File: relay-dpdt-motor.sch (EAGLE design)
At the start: 4 parts, among them K1 4052

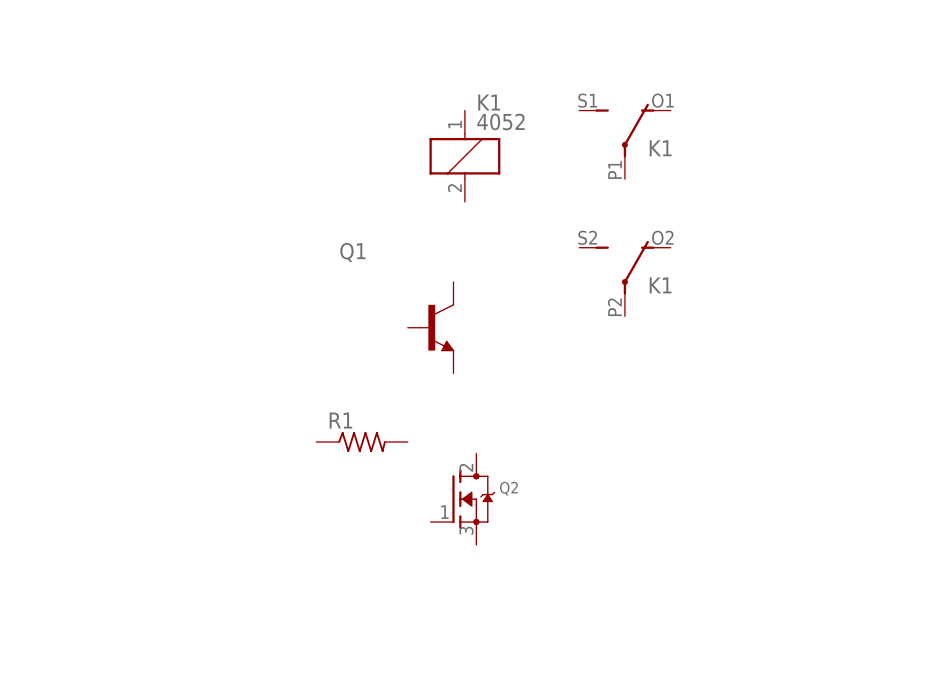
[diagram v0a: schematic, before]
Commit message: eagle prewired
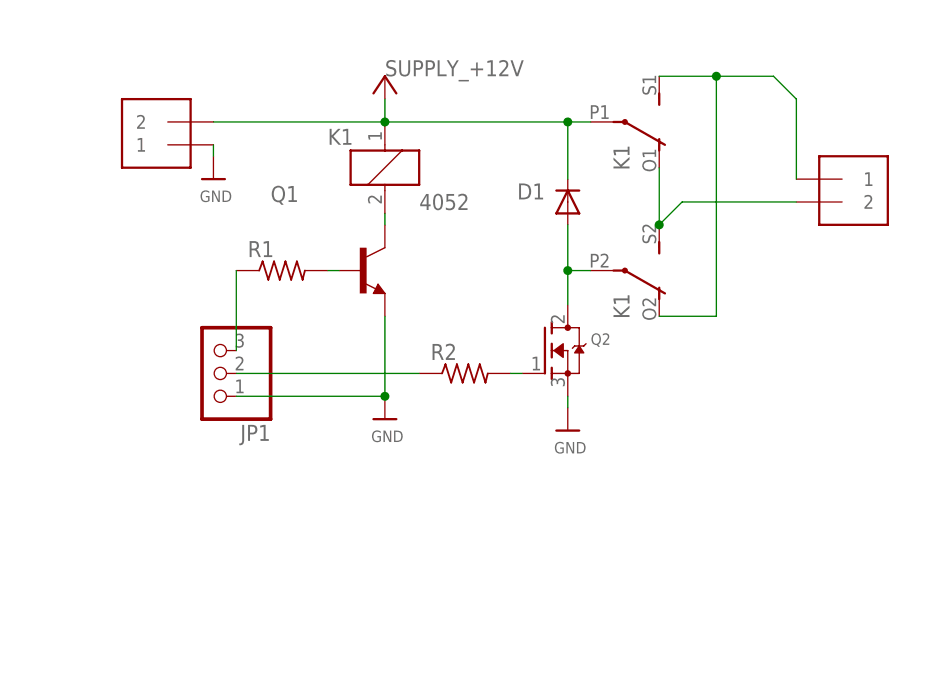
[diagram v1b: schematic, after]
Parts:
- added D1: 1N4004, adafruit:1N4004
- added J1, J2: 1X2-3.5MM, adafruit:1X2-3.5MM
- added JP1: (no value), adafruit:PINHD-1X3CB
- added R2: (no value), adafruit:R-US_0204/7
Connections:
- new net +12V: D1.C, J1.2, K11.1, K12.P
- new net GND: J1.1, JP1.1, Q1.E, Q2.S
- new net N$1: Q1.B, R1.2
- new net N$2: K11.2, Q1.C
- new net N$3: Q2.G, R2.2
- new net N$5: D1.A, K13.P, Q2.D
- new net N$6: J2.1, K12.S, K13.O
- new net N$7: J2.2, K12.O, K13.S
- new net N$8: JP1.2, R2.1
- new net N$9: JP1.3, R1.1
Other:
- moved on the sheet: K1, Q1, Q2, R1
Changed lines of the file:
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@@
 <setting verticaltext="up"/>
 </settings>
-<grid distance="0.1" unitdist="inch" unit="inch" style="lines" multiple="1" display="no" altdistance="0.01" altunitdist="inch" altunit="inch"/>
+<grid distance="50" unitdist="mil" unit="mil" style="lines" multiple="1" display="no" altdistance="25" altunitdist="mil" altunit="mil"/>
 <layers>
 <layer number="1" name="Top" color="4" fill="1" visible="no" active="no"/>
@@
 <part name="R1" library="adafruit" deviceset="R-US_" device="0204/7"/>
 <part name="Q2" library="adafruit" deviceset="MOSFET-N" device="GDS_TO220V"/>
+<part name="D1" library="adafruit" deviceset="1N4004" device=""/>
+<part name="J1" library="adafruit" deviceset="1X2" device="-3.5MM"/>
+<part name="+12V1" library="dp_devices" deviceset="SUPPLY_+12V" device=""/>
+<part name="R2" library="adafruit" deviceset="R-US_" device="0204/7"/>
+<part name="U$2" library="microbuilder" deviceset="GND" device=""/>
+<part name="J2" library="adafruit" deviceset="1X2" device="-3.5MM"/>
+<part name="JP1" library="adafruit" deviceset="PINHD-1X3" device="CB"/>
+<part name="U$3" library="microbuilder" deviceset="GND" device=""/>
+<part name="U$1" library="microbuilder" deviceset="GND" device=""/>
 </parts>
 <sheets>
@@
 </plain>
 <instances>
-<instance part="K1" gate="1" x="34.29" y="76.2"/>
-<instance part="K1" gate="2" x="52.07" y="76.2"/>
-<instance part="K1" gate="3" x="52.07" y="60.96"/>
-<instance part="Q1" gate="Q" x="30.48" y="57.15"/>
-<instance part="R1" gate="G$1" x="22.86" y="44.45"/>
-<instance part="Q2" gate="G$1" x="33.02" y="38.1"/>
+<instance part="K1" gate="1" x="25.4" y="74.93" smashed="yes">
+<attribute name="VALUE" x="29.21" y="70.231" size="1.778" layer="96"/>
+<attribute name="PART" x="19.05" y="77.47" size="1.778" layer="95"/>
+</instance>
+<instance part="K1" gate="2" x="50.8" y="80.01" smashed="yes" rot="R270">
+<attribute name="PART" x="50.8" y="77.47" size="1.778" layer="95" rot="R270"/>
+</instance>
+<instance part="K1" gate="3" x="50.8" y="63.5" smashed="yes" rot="R270">
+<attribute name="PART" x="50.8" y="60.96" size="1.778" layer="95" rot="R270"/>
+</instance>
+<instance part="Q1" gate="Q" x="22.86" y="63.5"/>
+<instance part="R1" gate="G$1" x="13.97" y="63.5"/>
+<instance part="Q2" gate="G$1" x="43.18" y="54.61"/>
+<instance part="D1" gate="1" x="45.72" y="71.12" smashed="yes" rot="R90">
+<attribute name="NAME" x="43.18" y="73.1774" size="1.778" layer="95" rot="R180"/>
+</instance>
+<instance part="J1" gate="G$1" x="1.27" y="80.01" rot="R180"/>
+<instance part="+12V1" gate="SUPPLY" x="25.4" y="82.55"/>
+<instance part="R2" gate="G$1" x="34.29" y="52.07"/>
+<instance part="U$2" gate="G$1" x="45.72" y="45.72"/>
+<instance part="J2" gate="G$1" x="76.2" y="71.12"/>
+<instance part="JP1" gate="A" x="6.35" y="52.07" rot="R180"/>
+<instance part="U$3" gate="G$1" x="25.4" y="46.99"/>
+<instance part="U$1" gate="G$1" x="6.35" y="73.66"/>
 </instances>
 <busses>
 </busses>
 <nets>
+<net name="N$1" class="0">
+<segment>
+<pinref part="Q1" gate="Q" pin="B"/>
+<pinref part="R1" gate="G$1" pin="2"/>
+<wire x1="19.05" y1="63.5" x2="20.32" y2="63.5" width="0.1524" layer="91"/>
+</segment>
+</net>
+<net name="+12V" class="0">
+<segment>
+<pinref part="K1" gate="2" pin="P"/>
+<pinref part="D1" gate="1" pin="C"/>
+<wire x1="45.72" y1="80.01" x2="48.26" y2="80.01" width="0.1524" layer="91"/>
+<wire x1="45.72" y1="80.01" x2="45.72" y2="73.66" width="0.1524" layer="91"/>
+<junction x="45.72" y="80.01"/>
+<pinref part="+12V1" gate="SUPPLY" pin="+12V"/>
+<pinref part="K1" gate="1" pin="1"/>
+<wire x1="25.4" y1="82.55" x2="25.4" y2="80.01" width="0.1524" layer="91"/>
+<wire x1="45.72" y1="80.01" x2="25.4" y2="80.01" width="0.1524" layer="91"/>
+<junction x="25.4" y="80.01"/>
+<pinref part="J1" gate="G$1" pin="2"/>
+<wire x1="25.4" y1="80.01" x2="6.35" y2="80.01" width="0.1524" layer="91"/>
+</segment>
+</net>
+<net name="N$2" class="0">
+<segment>
+<pinref part="K1" gate="1" pin="2"/>
+<pinref part="Q1" gate="Q" pin="C"/>
+<wire x1="25.4" y1="69.85" x2="25.4" y2="68.58" width="0.1524" layer="91"/>
+</segment>
+</net>
+<net name="GND" class="0">
+<segment>
+<pinref part="Q2" gate="G$1" pin="S"/>
+<pinref part="U$2" gate="G$1" pin="GND"/>
+<wire x1="45.72" y1="49.53" x2="45.72" y2="48.26" width="0.1524" layer="91"/>
+</segment>
+<segment>
+<pinref part="U$3" gate="G$1" pin="GND"/>
+<pinref part="JP1" gate="A" pin="1"/>
+<wire x1="25.4" y1="49.53" x2="8.89" y2="49.53" width="0.1524" layer="91"/>
+<pinref part="Q1" gate="Q" pin="E"/>
+<wire x1="25.4" y1="58.42" x2="25.4" y2="49.53" width="0.1524" layer="91"/>
+<junction x="25.4" y="49.53"/>
+</segment>
+<segment>
+<pinref part="J1" gate="G$1" pin="1"/>
+<pinref part="U$1" gate="G$1" pin="GND"/>
+<wire x1="6.35" y1="77.47" x2="6.35" y2="76.2" width="0.1524" layer="91"/>
+</segment>
+</net>
+<net name="N$3" class="0">
+<segment>
+<pinref part="Q2" gate="G$1" pin="G"/>
+<pinref part="R2" gate="G$1" pin="2"/>
+<wire x1="39.37" y1="52.07" x2="40.64" y2="52.07" width="0.1524" layer="91"/>
+</segment>
+</net>
+<net name="N$5" class="0">
+<segment>
+<pinref part="K1" gate="3" pin="P"/>
+<wire x1="48.26" y1="63.5" x2="45.72" y2="63.5" width="0.1524" layer="91"/>
+<pinref part="Q2" gate="G$1" pin="D"/>
+<wire x1="45.72" y1="63.5" x2="45.72" y2="59.69" width="0.1524" layer="91"/>
+<pinref part="D1" gate="1" pin="A"/>
+<wire x1="45.72" y1="68.58" x2="45.72" y2="63.5" width="0.1524" layer="91"/>
+<junction x="45.72" y="63.5"/>
+</segment>
+</net>
+<net name="N$6" class="0">
+<segment>
+<pinref part="K1" gate="2" pin="S"/>
+<wire x1="55.88" y1="85.09" x2="62.23" y2="85.09" width="0.1524" layer="91"/>
+<wire x1="62.23" y1="85.09" x2="68.58" y2="85.09" width="0.1524" layer="91"/>
+<wire x1="68.58" y1="85.09" x2="71.12" y2="82.55" width="0.1524" layer="91"/>
+<pinref part="J2" gate="G$1" pin="1"/>
+<wire x1="71.12" y1="82.55" x2="71.12" y2="73.66" width="0.1524" layer="91"/>
+<pinref part="K1" gate="3" pin="O"/>
+<wire x1="55.88" y1="58.42" x2="62.23" y2="58.42" width="0.1524" layer="91"/>
+<wire x1="62.23" y1="58.42" x2="62.23" y2="85.09" width="0.1524" layer="91"/>
+<junction x="62.23" y="85.09"/>
+</segment>
+</net>
+<net name="N$7" class="0">
+<segment>
+<pinref part="J2" gate="G$1" pin="2"/>
+<pinref part="K1" gate="3" pin="S"/>
+<wire x1="71.12" y1="71.12" x2="58.42" y2="71.12" width="0.1524" layer="91"/>
+<wire x1="58.42" y1="71.12" x2="55.88" y2="68.58" width="0.1524" layer="91"/>
+<pinref part="K1" gate="2" pin="O"/>
+<wire x1="55.88" y1="74.93" x2="55.88" y2="68.58" width="0.1524" layer="91"/>
+<junction x="55.88" y="68.58"/>
+</segment>
+</net>
+<net name="N$8" class="0">
+<segment>
+<pinref part="R2" gate="G$1" pin="1"/>
+<pinref part="JP1" gate="A" pin="2"/>
+<wire x1="8.89" y1="52.07" x2="29.21" y2="52.07" width="0.1524" layer="91"/>
+</segment>
+</net>
+<net name="N$9" class="0">
+<segment>
+<pinref part="R1" gate="G$1" pin="1"/>
+<pinref part="JP1" gate="A" pin="3"/>
+<wire x1="8.89" y1="63.5" x2="8.89" y2="54.61" width="0.1524" layer="91"/>
+</segment>
+</net>
 </nets>
 </sheet>

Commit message: with pnp
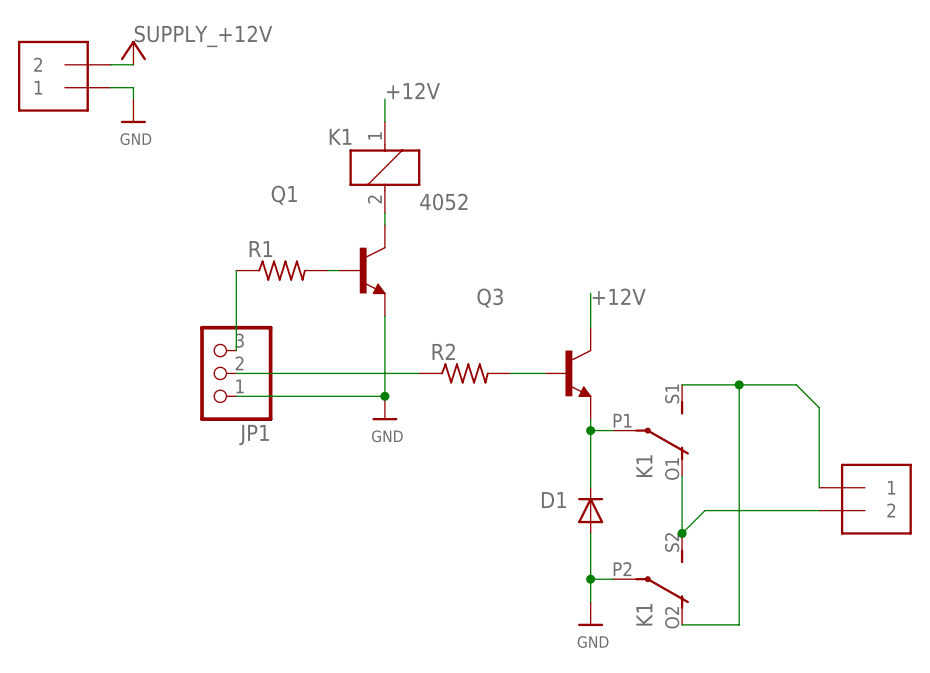
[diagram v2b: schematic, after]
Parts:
- removed Q2: (no value), adafruit:MOSFET-NGDS_TO220V
- added Q3: (no value), dp_devices:TRANSISTOR_BJT_NPN-TO-92-EBC
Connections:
- removed net N$5: D1.A, K13.P, Q2.D
- new net N$4: D1.C, K12.P, Q3.E
- net +12V: now also Q3.C; no longer D1.C, K12.P
- net GND: now also D1.A, K13.P; no longer Q2.S
- net N$3: now also Q3.B; no longer Q2.G
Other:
- moved on the sheet: D1, K1
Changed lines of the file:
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@@
 <part name="Q1" library="dp_devices" deviceset="TRANSISTOR_BJT_NPN" device="-TO-92-EBC"/>
 <part name="R1" library="adafruit" deviceset="R-US_" device="0204/7"/>
-<part name="Q2" library="adafruit" deviceset="MOSFET-N" device="GDS_TO220V"/>
 <part name="D1" library="adafruit" deviceset="1N4004" device=""/>
 <part name="J1" library="adafruit" deviceset="1X2" device="-3.5MM"/>
-<part name="+12V1" library="dp_devices" deviceset="SUPPLY_+12V" device=""/>
 <part name="R2" library="adafruit" deviceset="R-US_" device="0204/7"/>
 <part name="U$2" library="microbuilder" deviceset="GND" device=""/>
@@
 <part name="U$3" library="microbuilder" deviceset="GND" device=""/>
 <part name="U$1" library="microbuilder" deviceset="GND" device=""/>
+<part name="Q3" library="dp_devices" deviceset="TRANSISTOR_BJT_NPN" device="-TO-92-EBC"/>
+<part name="+12V2" library="dp_devices" deviceset="SUPPLY_+12V" device=""/>
 </parts>
 <sheets>
@@
 <attribute name="PART" x="19.05" y="77.47" size="1.778" layer="95"/>
 </instance>
-<instance part="K1" gate="2" x="50.8" y="80.01" smashed="yes" rot="R270">
-<attribute name="PART" x="50.8" y="77.47" size="1.778" layer="95" rot="R270"/>
+<instance part="K1" gate="2" x="53.34" y="45.72" smashed="yes" rot="R270">
+<attribute name="PART" x="53.34" y="43.18" size="1.778" layer="95" rot="R270"/>
 </instance>
-<instance part="K1" gate="3" x="50.8" y="63.5" smashed="yes" rot="R270">
-<attribute name="PART" x="50.8" y="60.96" size="1.778" layer="95" rot="R270"/>
+<instance part="K1" gate="3" x="53.34" y="29.21" smashed="yes" rot="R270">
+<attribute name="PART" x="53.34" y="26.67" size="1.778" layer="95" rot="R270"/>
 </instance>
 <instance part="Q1" gate="Q" x="22.86" y="63.5"/>
 <instance part="R1" gate="G$1" x="13.97" y="63.5"/>
-<instance part="Q2" gate="G$1" x="43.18" y="54.61"/>
-<instance part="D1" gate="1" x="45.72" y="71.12" smashed="yes" rot="R90">
-<attribute name="NAME" x="43.18" y="73.1774" size="1.778" layer="95" rot="R180"/>
+<instance part="D1" gate="1" x="48.26" y="36.83" smashed="yes" rot="R90">
+<attribute name="NAME" x="45.72" y="38.8874" size="1.778" layer="95" rot="R180"/>
 </instance>
-<instance part="J1" gate="G$1" x="1.27" y="80.01" rot="R180"/>
-<instance part="+12V1" gate="SUPPLY" x="25.4" y="82.55"/>
+<instance part="J1" gate="G$1" x="-10.16" y="86.36" rot="R180"/>
 <instance part="R2" gate="G$1" x="34.29" y="52.07"/>
-<instance part="U$2" gate="G$1" x="45.72" y="45.72"/>
-<instance part="J2" gate="G$1" x="76.2" y="71.12"/>
+<instance part="U$2" gate="G$1" x="48.26" y="24.13"/>
+<instance part="J2" gate="G$1" x="78.74" y="36.83"/>
 <instance part="JP1" gate="A" x="6.35" y="52.07" rot="R180"/>
 <instance part="U$3" gate="G$1" x="25.4" y="46.99"/>
-<instance part="U$1" gate="G$1" x="6.35" y="73.66"/>
+<instance part="U$1" gate="G$1" x="-2.54" y="80.01"/>
+<instance part="Q3" gate="Q" x="45.72" y="52.07"/>
+<instance part="+12V2" gate="SUPPLY" x="-2.54" y="86.36"/>
 </instances>
 <busses>
@@
 <net name="+12V" class="0">
 <segment>
-<pinref part="K1" gate="2" pin="P"/>
-<pinref part="D1" gate="1" pin="C"/>
-<wire x1="45.72" y1="80.01" x2="48.26" y2="80.01" width="0.1524" layer="91"/>
-<wire x1="45.72" y1="80.01" x2="45.72" y2="73.66" width="0.1524" layer="91"/>
-<junction x="45.72" y="80.01"/>
-<pinref part="+12V1" gate="SUPPLY" pin="+12V"/>
+<pinref part="J1" gate="G$1" pin="2"/>
+<pinref part="+12V2" gate="SUPPLY" pin="+12V"/>
+<wire x1="-2.54" y1="86.36" x2="-5.08" y2="86.36" width="0.1524" layer="91"/>
+</segment>
+<segment>
 <pinref part="K1" gate="1" pin="1"/>
 <wire x1="25.4" y1="82.55" x2="25.4" y2="80.01" width="0.1524" layer="91"/>
-<wire x1="45.72" y1="80.01" x2="25.4" y2="80.01" width="0.1524" layer="91"/>
-<junction x="25.4" y="80.01"/>
-<pinref part="J1" gate="G$1" pin="2"/>
-<wire x1="25.4" y1="80.01" x2="6.35" y2="80.01" width="0.1524" layer="91"/>
+<label x="25.4" y="82.55" size="1.778" layer="95"/>
+</segment>
+<segment>
+<pinref part="Q3" gate="Q" pin="C"/>
+<wire x1="48.26" y1="57.15" x2="48.26" y2="60.96" width="0.1524" layer="91"/>
+<label x="48.26" y="59.69" size="1.778" layer="95"/>
 </segment>
 </net>
@@
 <net name="GND" class="0">
 <segment>
-<pinref part="Q2" gate="G$1" pin="S"/>
 <pinref part="U$2" gate="G$1" pin="GND"/>
-<wire x1="45.72" y1="49.53" x2="45.72" y2="48.26" width="0.1524" layer="91"/>
+<pinref part="K1" gate="3" pin="P"/>
+<wire x1="50.8" y1="29.21" x2="48.26" y2="29.21" width="0.1524" layer="91"/>
+<pinref part="D1" gate="1" pin="A"/>
+<wire x1="48.26" y1="34.29" x2="48.26" y2="29.21" width="0.1524" layer="91"/>
+<wire x1="48.26" y1="29.21" x2="48.26" y2="26.67" width="0.1524" layer="91"/>
+<junction x="48.26" y="29.21"/>
 </segment>
 <segment>
@@
 <pinref part="J1" gate="G$1" pin="1"/>
 <pinref part="U$1" gate="G$1" pin="GND"/>
-<wire x1="6.35" y1="77.47" x2="6.35" y2="76.2" width="0.1524" layer="91"/>
+<wire x1="-5.08" y1="83.82" x2="-2.54" y2="83.82" width="0.1524" layer="91"/>
+<wire x1="-2.54" y1="83.82" x2="-2.54" y2="82.55" width="0.1524" layer="91"/>
 </segment>
 </net>
 <net name="N$3" class="0">
 <segment>
-<pinref part="Q2" gate="G$1" pin="G"/>
 <pinref part="R2" gate="G$1" pin="2"/>
-<wire x1="39.37" y1="52.07" x2="40.64" y2="52.07" width="0.1524" layer="91"/>
-</segment>
-</net>
-<net name="N$5" class="0">
-<segment>
-<pinref part="K1" gate="3" pin="P"/>
-<wire x1="48.26" y1="63.5" x2="45.72" y2="63.5" width="0.1524" layer="91"/>
-<pinref part="Q2" gate="G$1" pin="D"/>
-<wire x1="45.72" y1="63.5" x2="45.72" y2="59.69" width="0.1524" layer="91"/>
-<pinref part="D1" gate="1" pin="A"/>
-<wire x1="45.72" y1="68.58" x2="45.72" y2="63.5" width="0.1524" layer="91"/>
-<junction x="45.72" y="63.5"/>
+<wire x1="39.37" y1="52.07" x2="43.18" y2="52.07" width="0.1524" layer="91"/>
+<pinref part="Q3" gate="Q" pin="B"/>
 </segment>
 </net>
@@
 <segment>
 <pinref part="K1" gate="2" pin="S"/>
-<wire x1="55.88" y1="85.09" x2="62.23" y2="85.09" width="0.1524" layer="91"/>
-<wire x1="62.23" y1="85.09" x2="68.58" y2="85.09" width="0.1524" layer="91"/>
-<wire x1="68.58" y1="85.09" x2="71.12" y2="82.55" width="0.1524" layer="91"/>
+<wire x1="58.42" y1="50.8" x2="64.77" y2="50.8" width="0.1524" layer="91"/>
+<wire x1="64.77" y1="50.8" x2="71.12" y2="50.8" width="0.1524" layer="91"/>
+<wire x1="71.12" y1="50.8" x2="73.66" y2="48.26" width="0.1524" layer="91"/>
 <pinref part="J2" gate="G$1" pin="1"/>
-<wire x1="71.12" y1="82.55" x2="71.12" y2="73.66" width="0.1524" layer="91"/>
+<wire x1="73.66" y1="48.26" x2="73.66" y2="39.37" width="0.1524" layer="91"/>
 <pinref part="K1" gate="3" pin="O"/>
-<wire x1="55.88" y1="58.42" x2="62.23" y2="58.42" width="0.1524" layer="91"/>
-<wire x1="62.23" y1="58.42" x2="62.23" y2="85.09" width="0.1524" layer="91"/>
-<junction x="62.23" y="85.09"/>
+<wire x1="58.42" y1="24.13" x2="64.77" y2="24.13" width="0.1524" layer="91"/>
+<wire x1="64.77" y1="24.13" x2="64.77" y2="50.8" width="0.1524" layer="91"/>
+<junction x="64.77" y="50.8"/>
 </segment>
 </net>
@@
 <pinref part="J2" gate="G$1" pin="2"/>
 <pinref part="K1" gate="3" pin="S"/>
-<wire x1="71.12" y1="71.12" x2="58.42" y2="71.12" width="0.1524" layer="91"/>
-<wire x1="58.42" y1="71.12" x2="55.88" y2="68.58" width="0.1524" layer="91"/>
+<wire x1="73.66" y1="36.83" x2="60.96" y2="36.83" width="0.1524" layer="91"/>
+<wire x1="60.96" y1="36.83" x2="58.42" y2="34.29" width="0.1524" layer="91"/>
 <pinref part="K1" gate="2" pin="O"/>
-<wire x1="55.88" y1="74.93" x2="55.88" y2="68.58" width="0.1524" layer="91"/>
-<junction x="55.88" y="68.58"/>
+<wire x1="58.42" y1="40.64" x2="58.42" y2="34.29" width="0.1524" layer="91"/>
+<junction x="58.42" y="34.29"/>
 </segment>
 </net>
@@
 </segment>
 </net>
+<net name="N$4" class="0">
+<segment>
+<pinref part="D1" gate="1" pin="C"/>
+<pinref part="K1" gate="2" pin="P"/>
+<wire x1="48.26" y1="45.72" x2="50.8" y2="45.72" width="0.1524" layer="91"/>
+<wire x1="48.26" y1="45.72" x2="48.26" y2="39.37" width="0.1524" layer="91"/>
+<pinref part="Q3" gate="Q" pin="E"/>
+<wire x1="48.26" y1="46.99" x2="48.26" y2="45.72" width="0.1524" layer="91"/>
+<junction x="48.26" y="45.72"/>
+</segment>
+</net>
